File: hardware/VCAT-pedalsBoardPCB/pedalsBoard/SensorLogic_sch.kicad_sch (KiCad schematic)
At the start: 33 parts, among them U2 Opamp_Dual, U3 Opamp_Dual

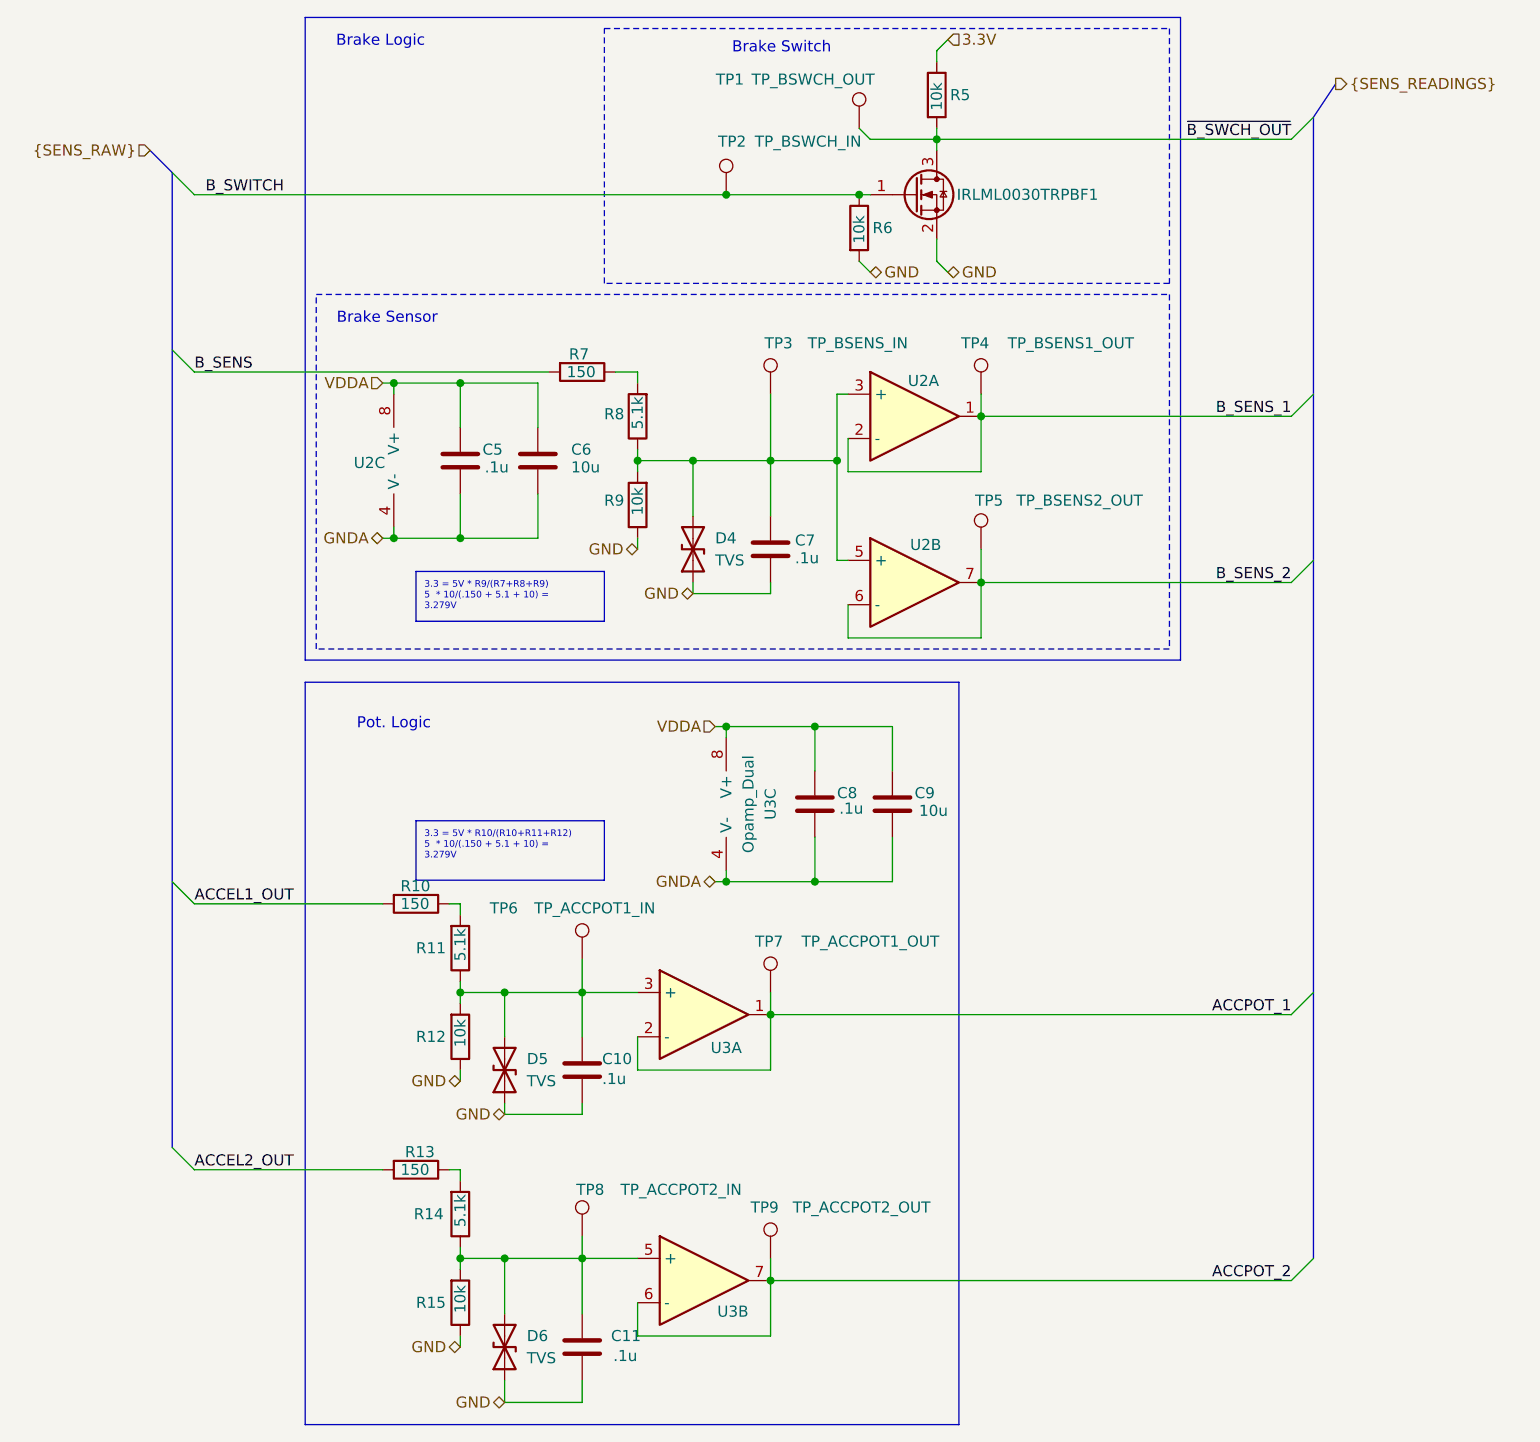
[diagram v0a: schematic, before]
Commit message: hopefully final before layout
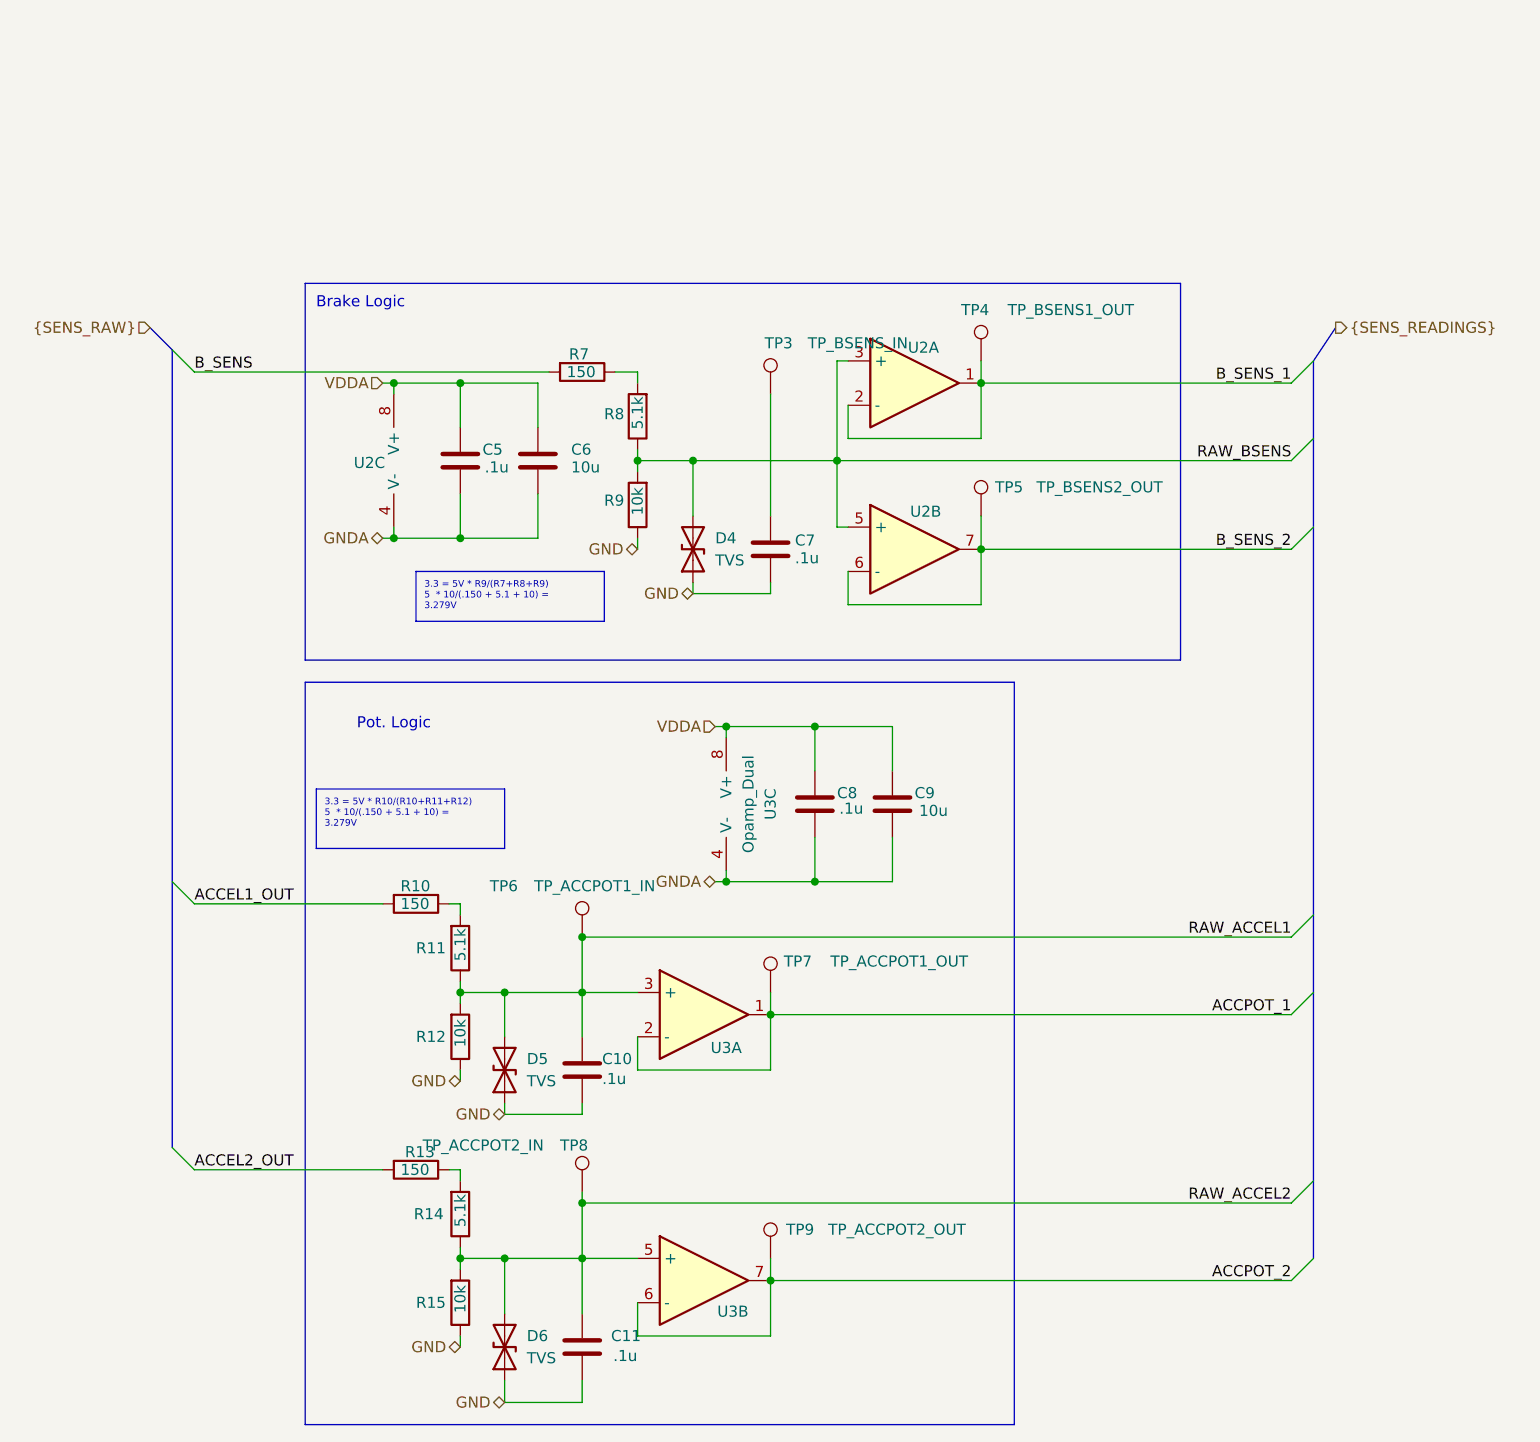
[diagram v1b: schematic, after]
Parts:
- removed IRLML0030TRPBF1: IRLML0030, SOT95P237X112-3N, symbol Transistor_FET:IRLML0030
- removed R5, R6: 10k, Resistor_SMD:R_0603_1608Metric_Pad0.98x0.95mm_HandSolder, symbol Device:R
- removed TP1: TP_BSWCH_OUT, symbol Connector:TestPoint
- removed TP2: TP_BSWCH_IN, symbol Connector:TestPoint
- C10, C11, C7: footprint SD15C01FTG -> Capacitor_SMD:C_0603_1608Metric_Pad1.08x0.95mm_HandSolder
- D4, D5, D6: footprint MyParts:SD15C01FTG -> Diode_SMD:D_SOD-323
- TP3, TP4, TP5, TP6, TP7, TP8, TP9: footprint (none) -> LHRS_Special:TestPoint_HEX_3mmID
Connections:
- net RAW_ACCEL1: now reaches C10.1, D5.2 (A2), R11.1, R12.2, TP6.1, U3.3 (+)
- net RAW_BSENS: now reaches D4.2 (A2), R8.1, R9.2, U2.3 (+), U2.5 (+)
- net RAW_BSENS: no longer C7.1, TP3.1
- net RAW_ACCEL2: now reaches C11.1, D6.2 (A2), R14.1, R15.2, TP8.1, U3.5 (+)
- new net: C7.1, TP3.1
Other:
- note removed: "Brake Sensor"
- note removed: "Brake Switch"
- moved on the sheet: TP4, TP5, TP6, TP8, U2A, U2B
